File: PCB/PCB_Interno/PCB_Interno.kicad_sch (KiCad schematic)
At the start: 5 parts, among them J2 Conn_02x24_Odd_Even

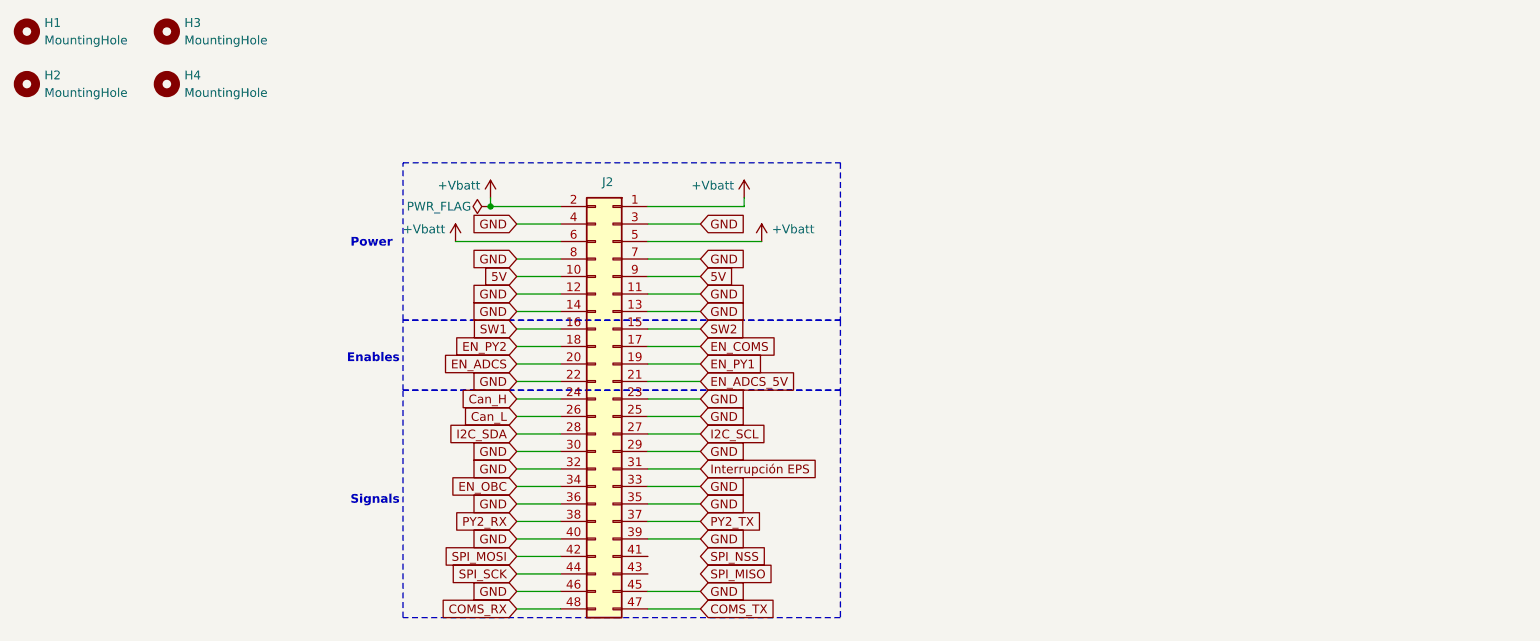
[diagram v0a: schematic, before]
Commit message: PC104
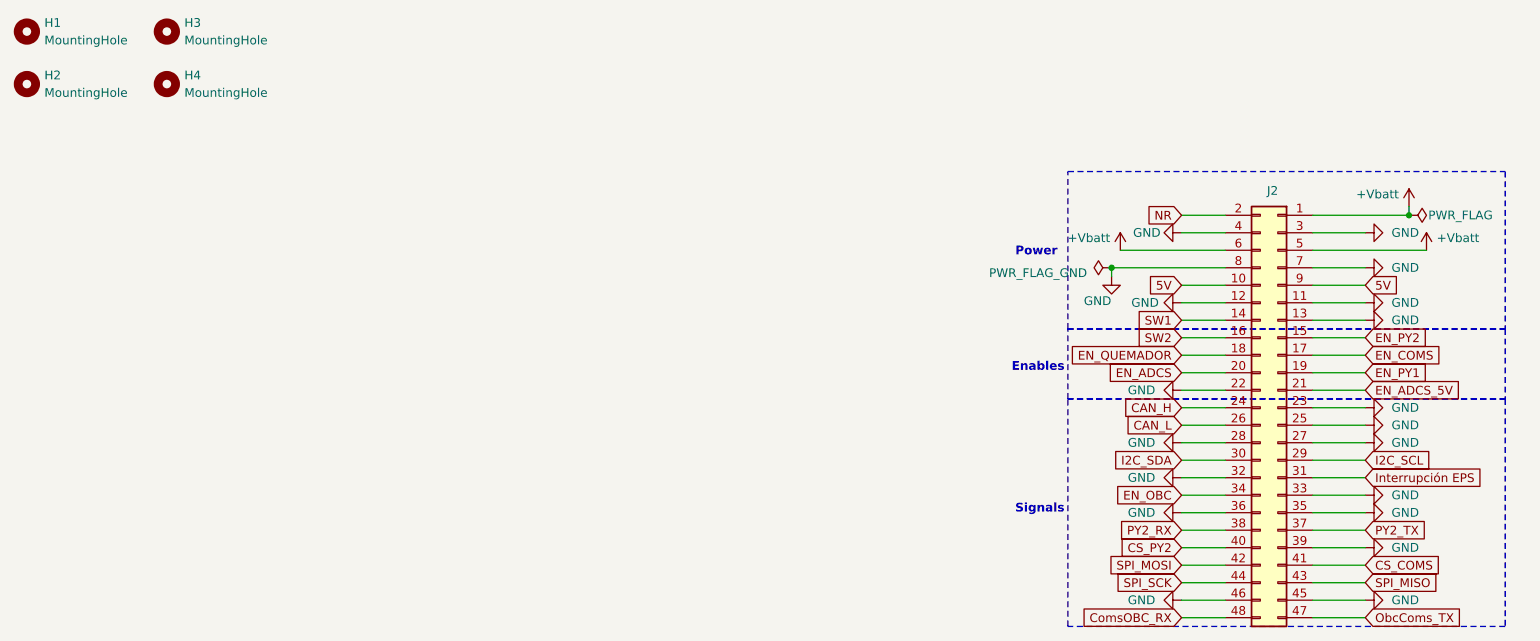
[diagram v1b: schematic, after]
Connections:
- net +Vbatt: no longer J2.2 (Pin_2)
- net EN_PY2: now also J2.15 (Pin_15); no longer J2.18 (Pin_18)
- net GND: now also J2.27 (Pin_27), J2.28 (Pin_28); no longer J2.14 (Pin_14), J2.29 (Pin_29), J2.30 (Pin_30), J2.40 (Pin_40)
- net I2C_SCL: now also J2.29 (Pin_29); no longer J2.27 (Pin_27)
- net I2C_SDA: now also J2.30 (Pin_30); no longer J2.28 (Pin_28)
- net SPI_MISO: now also J2.43 (Pin_43)
- net SW1: now also J2.14 (Pin_14); no longer J2.16 (Pin_16)
- net SW2: now also J2.16 (Pin_16); no longer J2.15 (Pin_15)
- net CS_COMS: now reaches J2.41 (Pin_41)
- net COMS_RX renamed ComsOBC_RX
- net COMS_TX renamed ObcComs_TX
- net Can_H renamed CAN_H
- net Can_L renamed CAN_L
- new net CS_PY2: J2.40 (Pin_40)
- new net EN_QUEMADOR: J2.18 (Pin_18)
- new net NR: J2.2 (Pin_2)
